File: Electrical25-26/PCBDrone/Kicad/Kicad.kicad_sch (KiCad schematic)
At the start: 35 parts, among them J1 Conn_01x02_Pin, J2 Conn_01x04, U1 ESP32-WROOM-32E, U2 BMI323, U3 DRV8210DSGR, U4 DRV8210DSGR, U5 DRV8210DSGR, U6 DRV8210DSGR

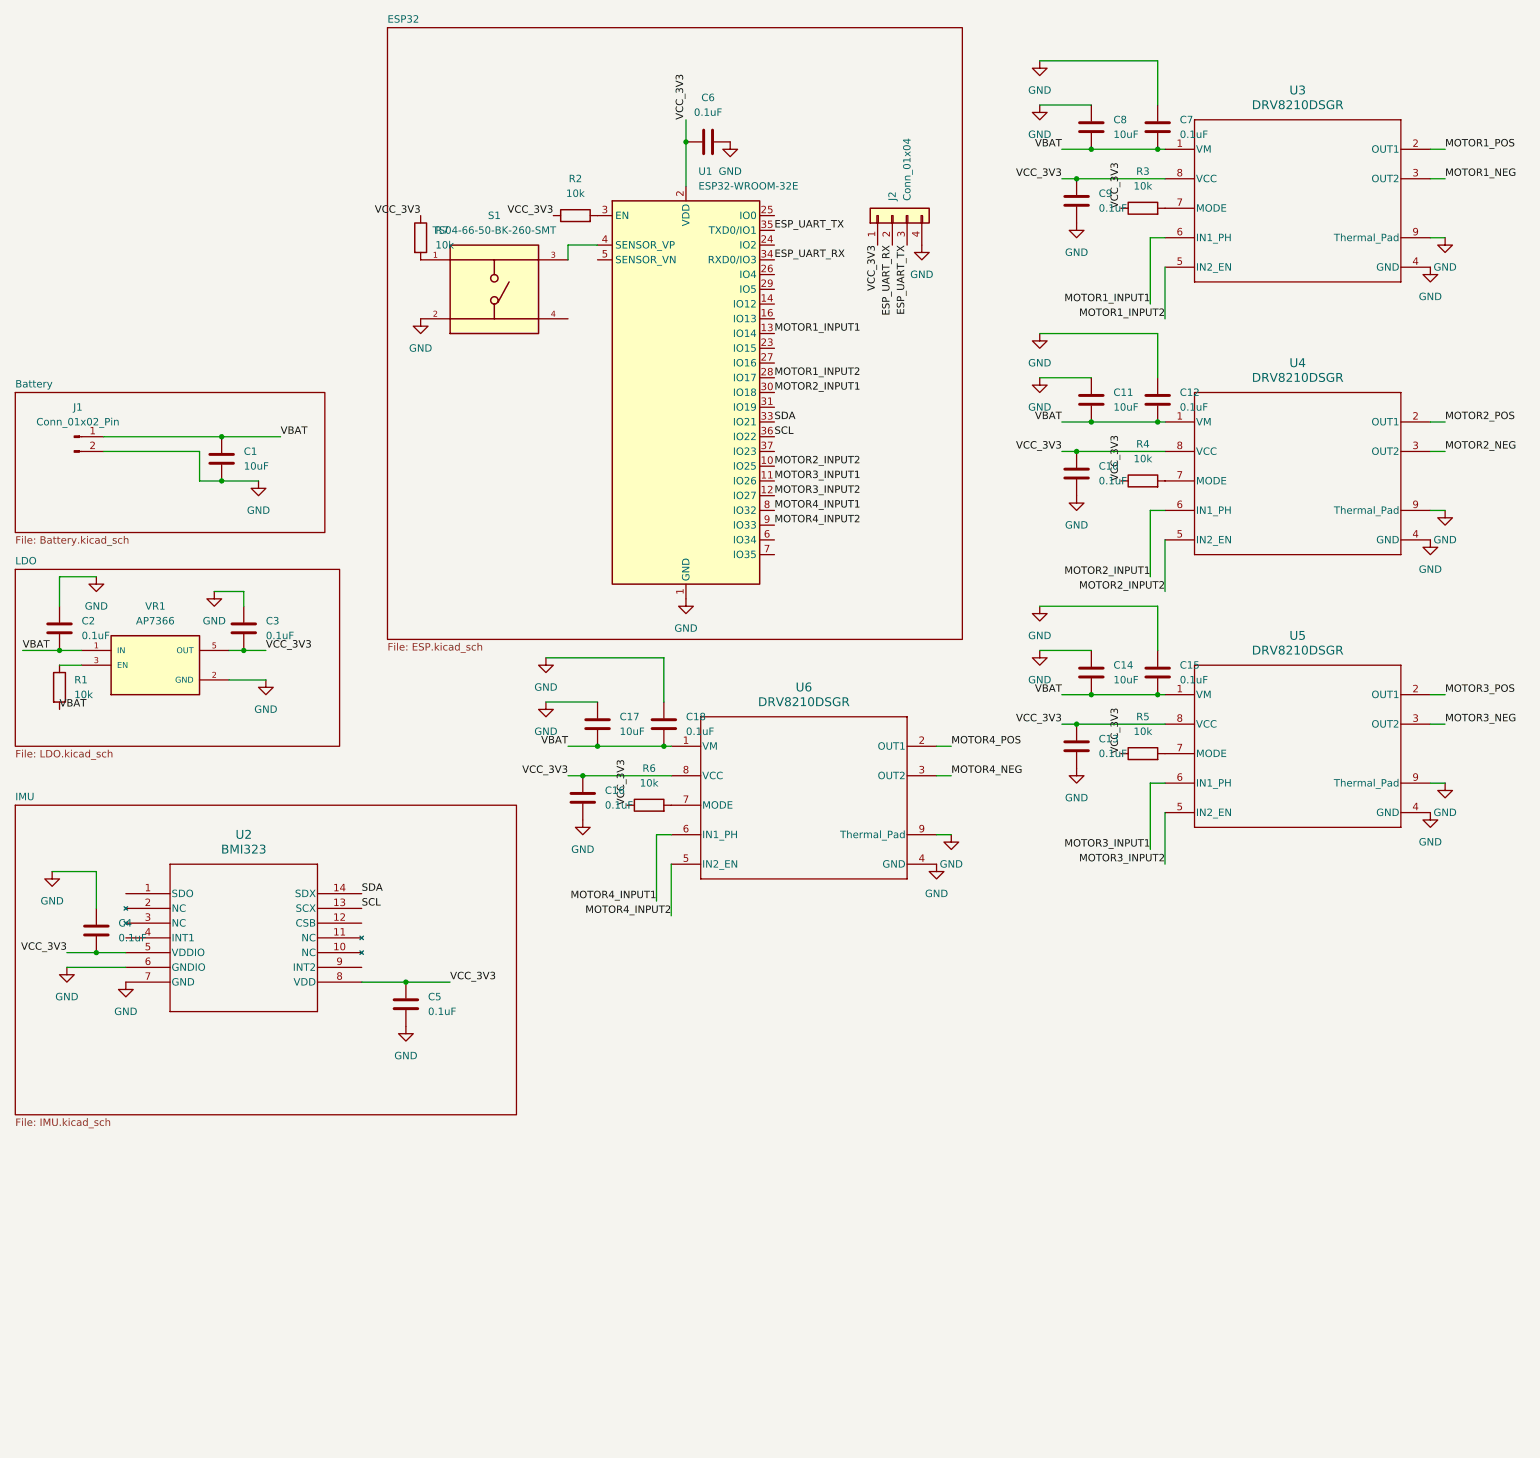
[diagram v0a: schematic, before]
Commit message: Everything done except logo and name
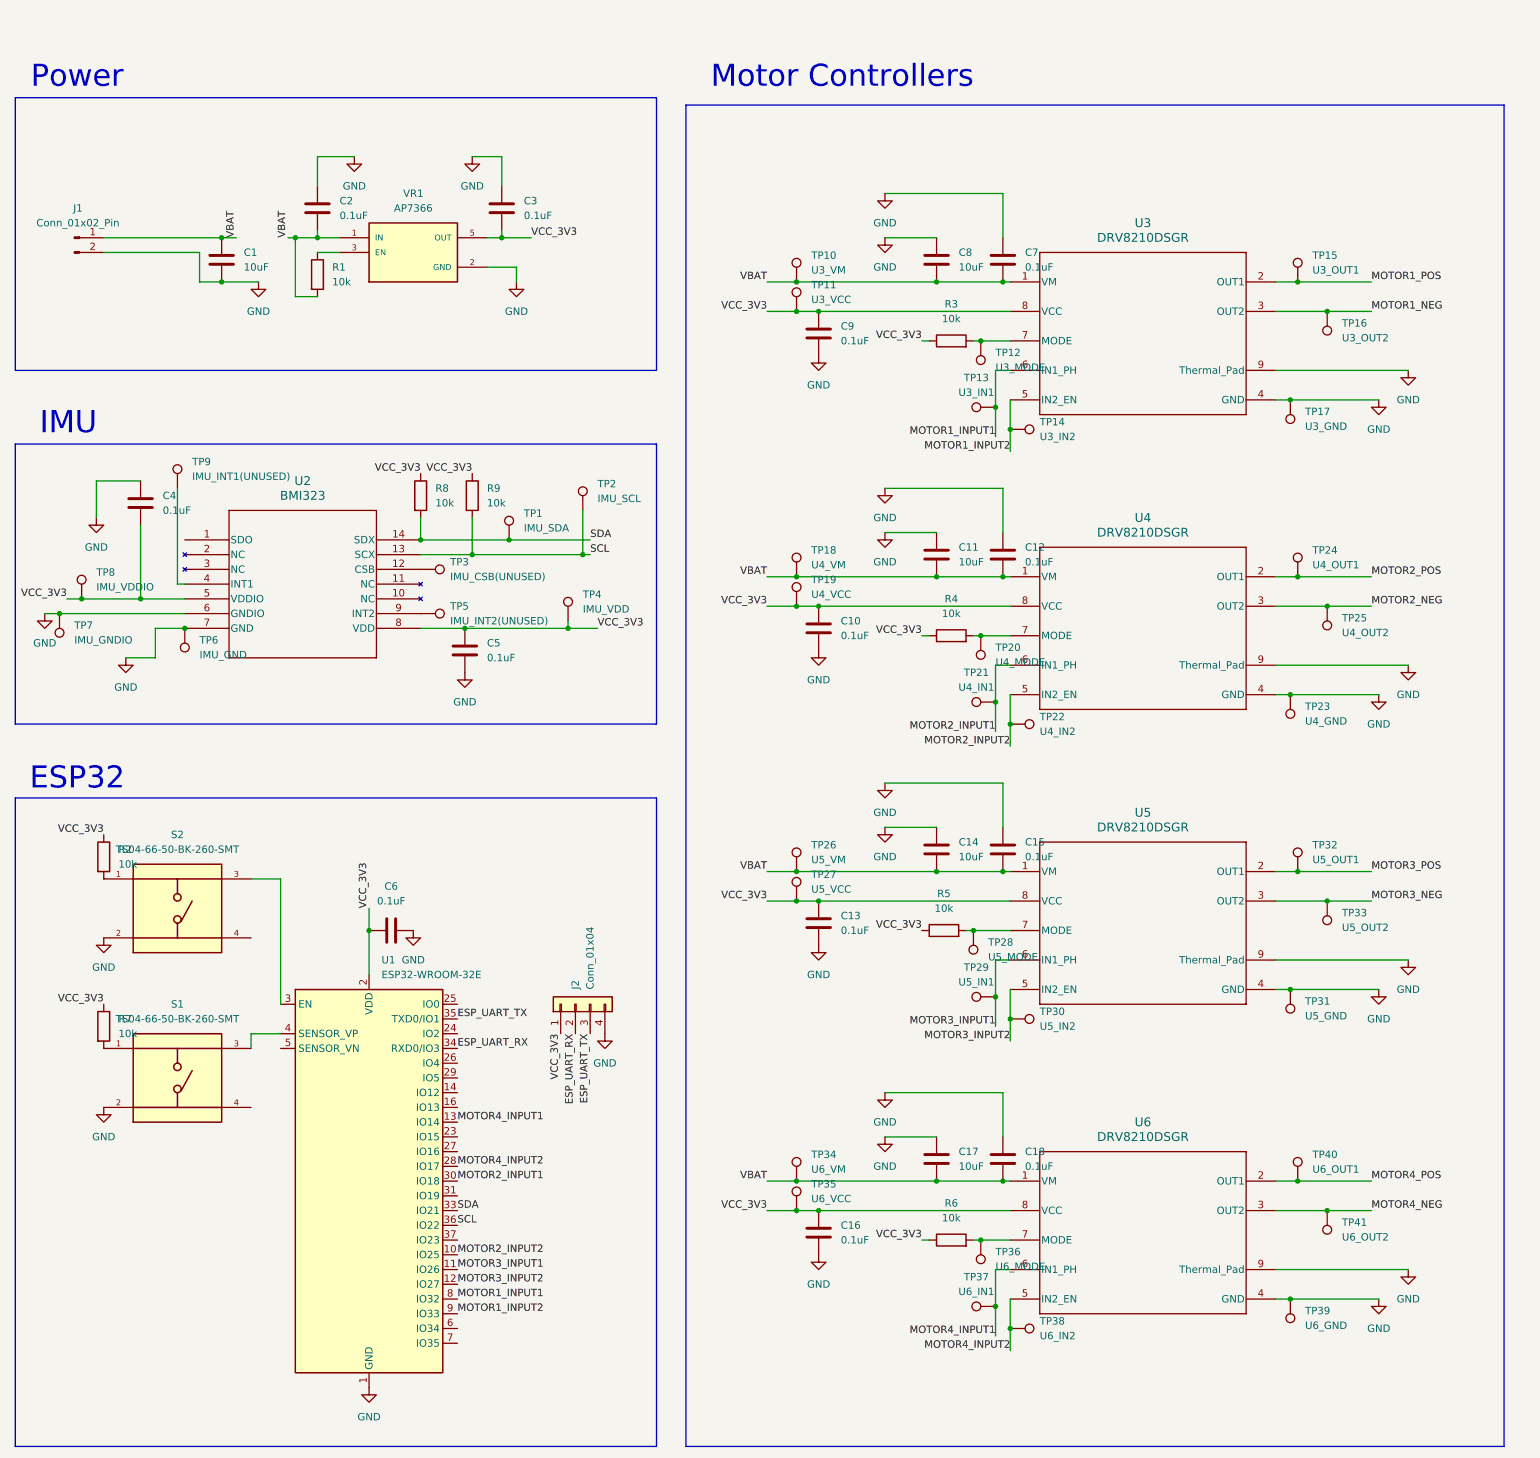
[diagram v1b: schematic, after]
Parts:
- added R8, R9: 10k, Resistor_SMD:R_0603_1608Metric, symbol Device:R
- added S2: TS04-66-50-BK-260-SMT, footprints:SW_TS04-66-50-BK-260-SMT, symbol TS04-66-50-BK-260-SMT:TS04-66-50-BK-260-SMT
- added TP1: IMU_SDA, TestPoint:TestPoint_Pad_1.0x1.0mm, symbol Connector:TestPoint
- added TP10: U3_VM, TestPoint:TestPoint_Pad_1.0x1.0mm, symbol Connector:TestPoint
- added TP11: U3_VCC, TestPoint:TestPoint_Pad_1.0x1.0mm, symbol Connector:TestPoint
- added TP12: U3_MODE, TestPoint:TestPoint_Pad_1.0x1.0mm, symbol Connector:TestPoint
- added TP13: U3_IN1, TestPoint:TestPoint_Pad_1.0x1.0mm, symbol Connector:TestPoint
- added TP14: U3_IN2, TestPoint:TestPoint_Pad_1.0x1.0mm, symbol Connector:TestPoint
- added TP15: U3_OUT1, TestPoint:TestPoint_Pad_1.0x1.0mm, symbol Connector:TestPoint
- added TP16: U3_OUT2, TestPoint:TestPoint_Pad_1.0x1.0mm, symbol Connector:TestPoint
- added TP17: U3_GND, TestPoint:TestPoint_Pad_1.0x1.0mm, symbol Connector:TestPoint
- added TP18: U4_VM, TestPoint:TestPoint_Pad_1.0x1.0mm, symbol Connector:TestPoint
- added TP19: U4_VCC, TestPoint:TestPoint_Pad_1.0x1.0mm, symbol Connector:TestPoint
- added TP2: IMU_SCL, TestPoint:TestPoint_Pad_1.0x1.0mm, symbol Connector:TestPoint
- added TP20: U4_MODE, TestPoint:TestPoint_Pad_1.0x1.0mm, symbol Connector:TestPoint
- added TP21: U4_IN1, TestPoint:TestPoint_Pad_1.0x1.0mm, symbol Connector:TestPoint
- added TP22: U4_IN2, TestPoint:TestPoint_Pad_1.0x1.0mm, symbol Connector:TestPoint
- added TP23: U4_GND, TestPoint:TestPoint_Pad_1.0x1.0mm, symbol Connector:TestPoint
- added TP24: U4_OUT1, TestPoint:TestPoint_Pad_1.0x1.0mm, symbol Connector:TestPoint
- added TP25: U4_OUT2, TestPoint:TestPoint_Pad_1.0x1.0mm, symbol Connector:TestPoint
- added TP26: U5_VM, TestPoint:TestPoint_Pad_1.0x1.0mm, symbol Connector:TestPoint
- added TP27: U5_VCC, TestPoint:TestPoint_Pad_1.0x1.0mm, symbol Connector:TestPoint
- added TP28: U5_MODE, TestPoint:TestPoint_Pad_1.0x1.0mm, symbol Connector:TestPoint
- added TP29: U5_IN1, TestPoint:TestPoint_Pad_1.0x1.0mm, symbol Connector:TestPoint
- added TP3: IMU_CSB(UNUSED), TestPoint:TestPoint_Pad_1.0x1.0mm, symbol Connector:TestPoint
- added TP30: U5_IN2, TestPoint:TestPoint_Pad_1.0x1.0mm, symbol Connector:TestPoint
- added TP31: U5_GND, TestPoint:TestPoint_Pad_1.0x1.0mm, symbol Connector:TestPoint
- added TP32: U5_OUT1, TestPoint:TestPoint_Pad_1.0x1.0mm, symbol Connector:TestPoint
- added TP33: U5_OUT2, TestPoint:TestPoint_Pad_1.0x1.0mm, symbol Connector:TestPoint
- added TP34: U6_VM, TestPoint:TestPoint_Pad_1.0x1.0mm, symbol Connector:TestPoint
- added TP35: U6_VCC, TestPoint:TestPoint_Pad_1.0x1.0mm, symbol Connector:TestPoint
- added TP36: U6_MODE, TestPoint:TestPoint_Pad_1.0x1.0mm, symbol Connector:TestPoint
- added TP37: U6_IN1, TestPoint:TestPoint_Pad_1.0x1.0mm, symbol Connector:TestPoint
- added TP38: U6_IN2, TestPoint:TestPoint_Pad_1.0x1.0mm, symbol Connector:TestPoint
- added TP39: U6_GND, TestPoint:TestPoint_Pad_1.0x1.0mm, symbol Connector:TestPoint
- added TP4: IMU_VDD, TestPoint:TestPoint_Pad_1.0x1.0mm, symbol Connector:TestPoint
- added TP40: U6_OUT1, TestPoint:TestPoint_Pad_1.0x1.0mm, symbol Connector:TestPoint
- added TP41: U6_OUT2, TestPoint:TestPoint_Pad_1.0x1.0mm, symbol Connector:TestPoint
- added TP5: IMU_INT2(UNUSED), TestPoint:TestPoint_Pad_1.0x1.0mm, symbol Connector:TestPoint
- added TP6: IMU_GND, TestPoint:TestPoint_Pad_1.0x1.0mm, symbol Connector:TestPoint
- added TP7: IMU_GNDIO, TestPoint:TestPoint_Pad_1.0x1.0mm, symbol Connector:TestPoint
- added TP8: IMU_VDDIO, TestPoint:TestPoint_Pad_1.0x1.0mm, symbol Connector:TestPoint
- added TP9: IMU_INT1(UNUSED), TestPoint:TestPoint_Pad_1.0x1.0mm, symbol Connector:TestPoint
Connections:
- net GND: now also S2.2, TP17.1, TP23.1, TP31.1, TP39.1, TP6.1, TP7.1
- net MOTOR1_INPUT1: now also U1.8 (IO32), TP13.1; no longer U1.13 (IO14)
- net MOTOR1_INPUT2: now also U1.9 (IO33), TP14.1; no longer U1.28 (IO17)
- net MOTOR1_NEG: now also TP16.1
- net MOTOR1_POS: now also TP15.1
- net MOTOR2_INPUT1: now also TP21.1
- net MOTOR2_INPUT2: now also TP22.1
- net MOTOR2_NEG: now also TP25.1
- net MOTOR2_POS: now also TP24.1
- net MOTOR3_INPUT1: now also TP29.1
- net MOTOR3_INPUT2: now also TP30.1
- net MOTOR3_NEG: now also TP33.1
- net MOTOR3_POS: now also TP32.1
- net MOTOR4_INPUT1: now also U1.13 (IO14), TP37.1; no longer U1.8 (IO32)
- net MOTOR4_INPUT2: now also U1.28 (IO17), TP38.1; no longer U1.9 (IO33)
- net MOTOR4_NEG: now also TP41.1
- net MOTOR4_POS: now also TP40.1
- net SCL: now also R9.2, TP2.1
- net SDA: now also R8.2, TP1.1
- net VBAT: now also TP10.1, TP18.1, TP26.1, TP34.1
- net VCC_3V3: now also R8.1, R9.1, TP11.1, TP19.1, TP27.1, TP35.1, TP4.1, TP8.1
- net at R3.2, U3.7 (MODE): now also TP12.1
- net at R6.2, U6.7 (MODE): now also TP36.1
- net at U1.3 (EN): now also S2.3; no longer R2.2
- net at R5.2, U5.7 (MODE): now also TP28.1
- net at R4.2, U4.7 (MODE): now also TP20.1
- net at U2.12 (CSB): now also TP3.1
- net at U2.4 (INT1): now also TP9.1
- net at U2.9 (INT2): now also TP5.1
- new net: R2.2, S2.1
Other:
- removed sheet Battery
- removed sheet ESP32
- removed sheet IMU
- removed sheet LDO
- note added: "ESP32"
- note added: "IMU"
- note added: "Motor Controllers"
- note added: "Power"
- moved on the sheet: C1, C2, C3, C4, C5, C6, C7, C8, C9, J1, J2, R1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
